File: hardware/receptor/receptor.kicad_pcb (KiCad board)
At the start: 2 copper layers, 100 x 76 mm, 48 parts, among them J1 I2C, J2 USB-C, J3 5V EXT, J4 BOBINA 5V, Q1 AO3400A, SW1 RESET, SW2 BOOT, U1 ESP32-C3-MINI-1-H4X, U2 E220-900T30D, U4 USBLC6-2SC6, U5 AP2112K-3.3

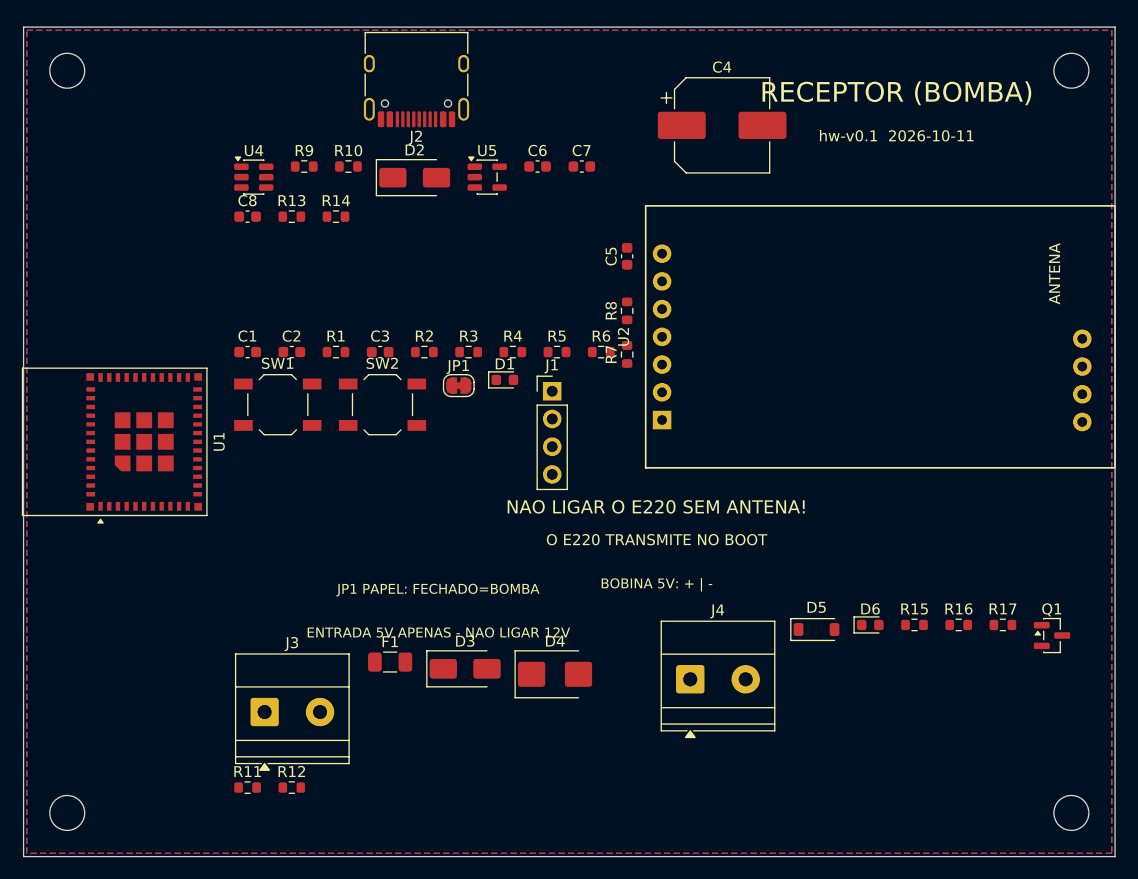
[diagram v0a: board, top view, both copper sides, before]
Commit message: feat(hw): layout compacto de 86x52 mm nas duas placas
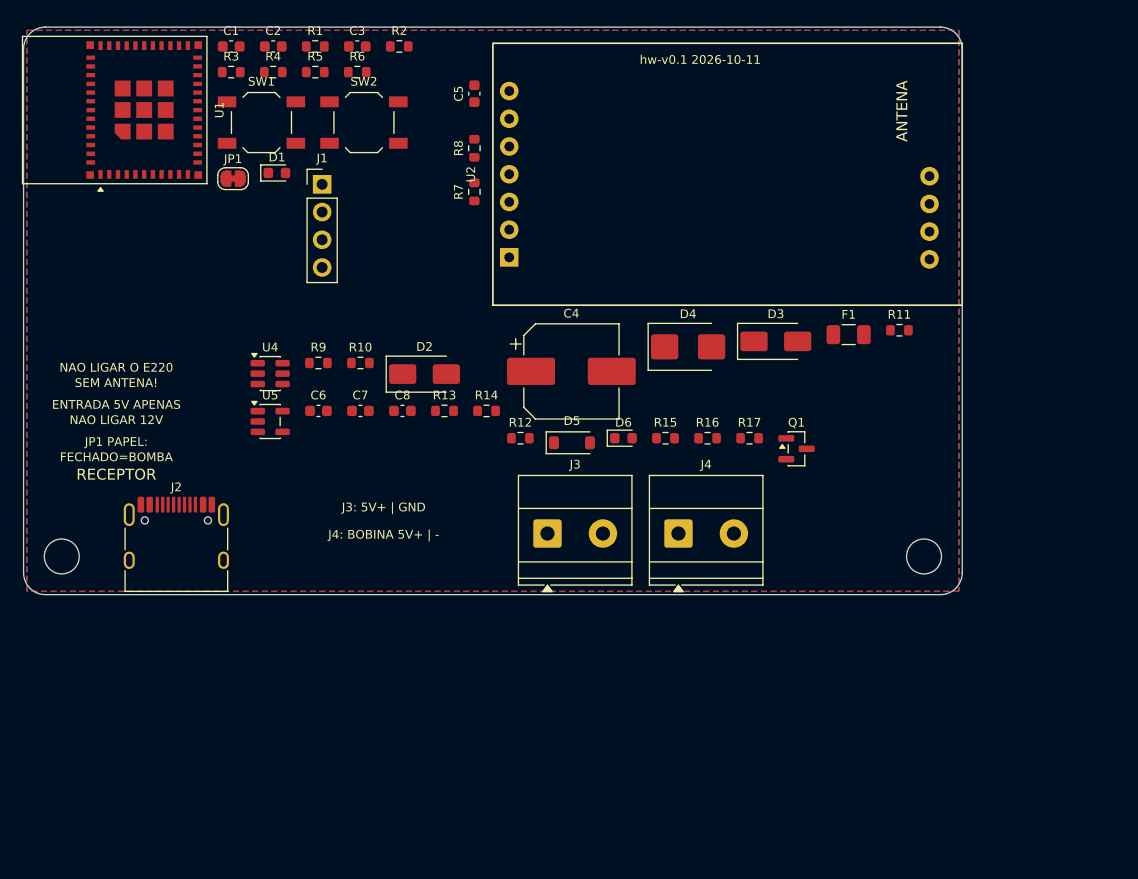
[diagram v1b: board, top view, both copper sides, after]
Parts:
- removed H3, H4: MountingHole_3.2mm_M3, MountingHole:MountingHole_3.2mm_M3
- moved R11 73.0 mm to (80.2, 27.8)
- moved F1 51.6 mm to (75.6, 28.2)
- moved J2 48.7 mm to (14.0, 47.8), turned to 0 degrees
- moved H2 46.5 mm to (82.5, 48.5)
- moved H1 44.5 mm to (3.50, 48.5)
- moved D3 41.4 mm to (68.9, 28.8)
- moved R12 38.3 mm to (45.5, 37.7)
- moved R6 34.0 mm to (30.6, 4.12)
- moved R5 33.9 mm to (26.7, 4.12)
- moved R4 33.8 mm to (22.9, 4.12)
- moved R3 33.6 mm to (19.0, 4.12)
- moved D4 32.4 mm to (60.9, 29.3)
- moved J3 30.6 mm to (48.0, 46.4)
- moved U1 30.4 mm to (11.1, 7.60)
- moved C7 30.2 mm to (30.9, 35.2)
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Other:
- board size 100 x 76 mm -> 86 x 52 mm
- board text added: "ENTRADA 5V APENAS"
- board text added: "FECHADO=BOMBA"
- board text added: "J3: 5V+ | GND"
- board text added: "J4: BOBINA 5V+ | -"
- board text added: "JP1 PAPEL:"
- board text added: "NAO LIGAR 12V"
- board text added: "NAO LIGAR O E220"
- board text added: "RECEPTOR"
- board text added: "SEM ANTENA!"
- board text removed: "BOBINA 5V: + | -"
- board text removed: "ENTRADA 5V APENAS - NAO LIGAR 12V"
- board text removed: "JP1 PAPEL: FECHADO=BOMBA"
- board text removed: "NAO LIGAR O E220 SEM ANTENA!"
- board text removed: "O E220 TRANSMITE NO BOOT"
- board text removed: "RECEPTOR (BOMBA)"
